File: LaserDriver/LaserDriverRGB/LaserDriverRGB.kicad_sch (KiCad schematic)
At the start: 15 parts

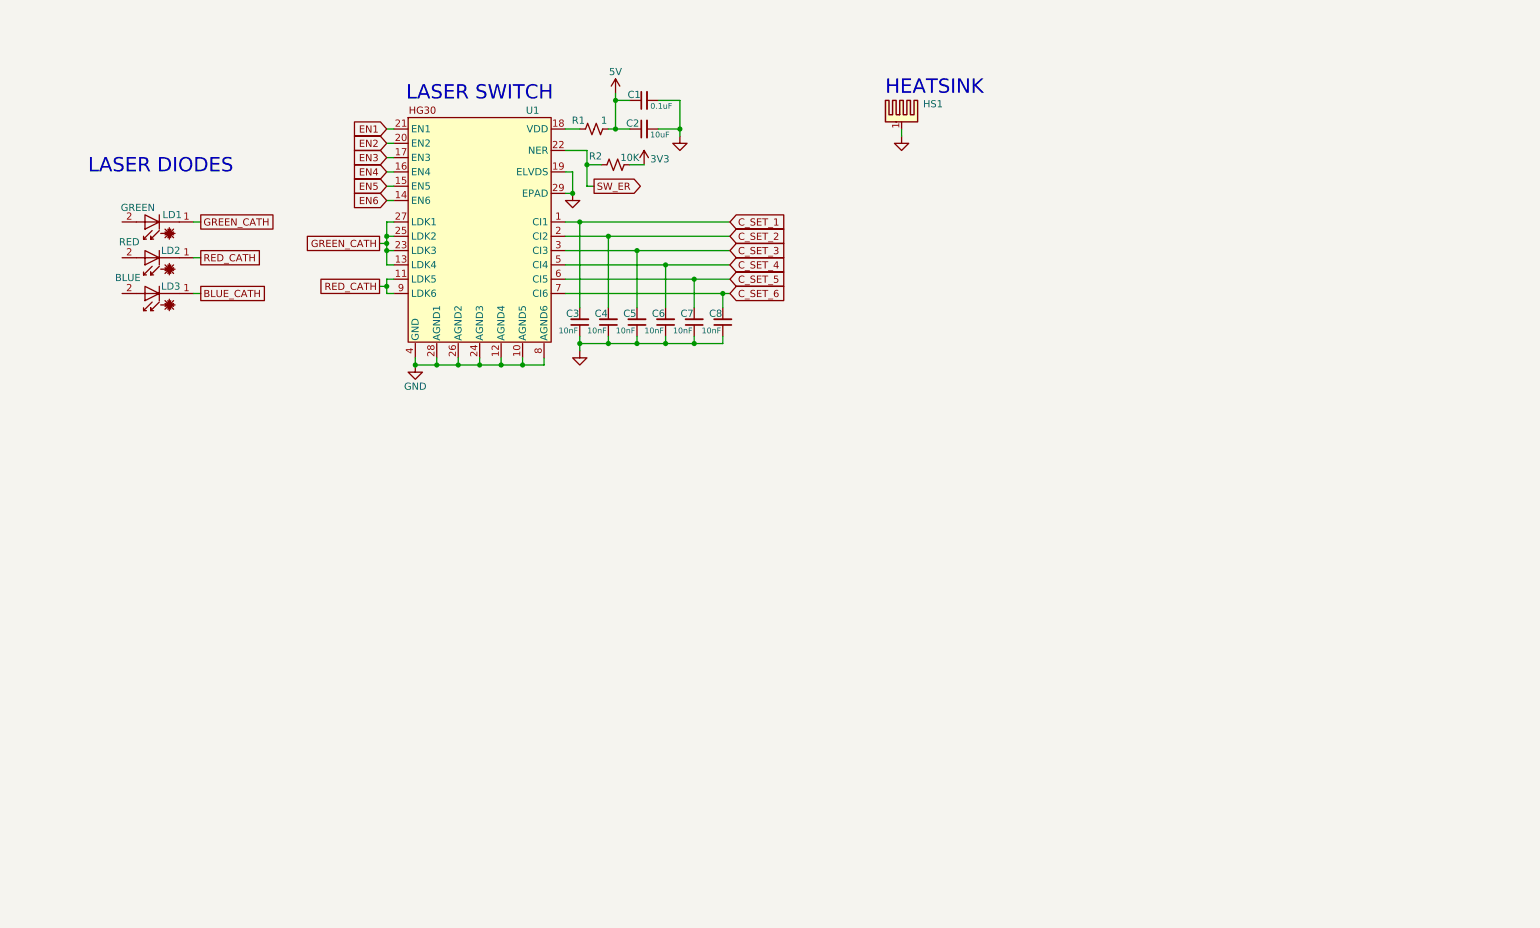
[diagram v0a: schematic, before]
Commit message: pcb chilling
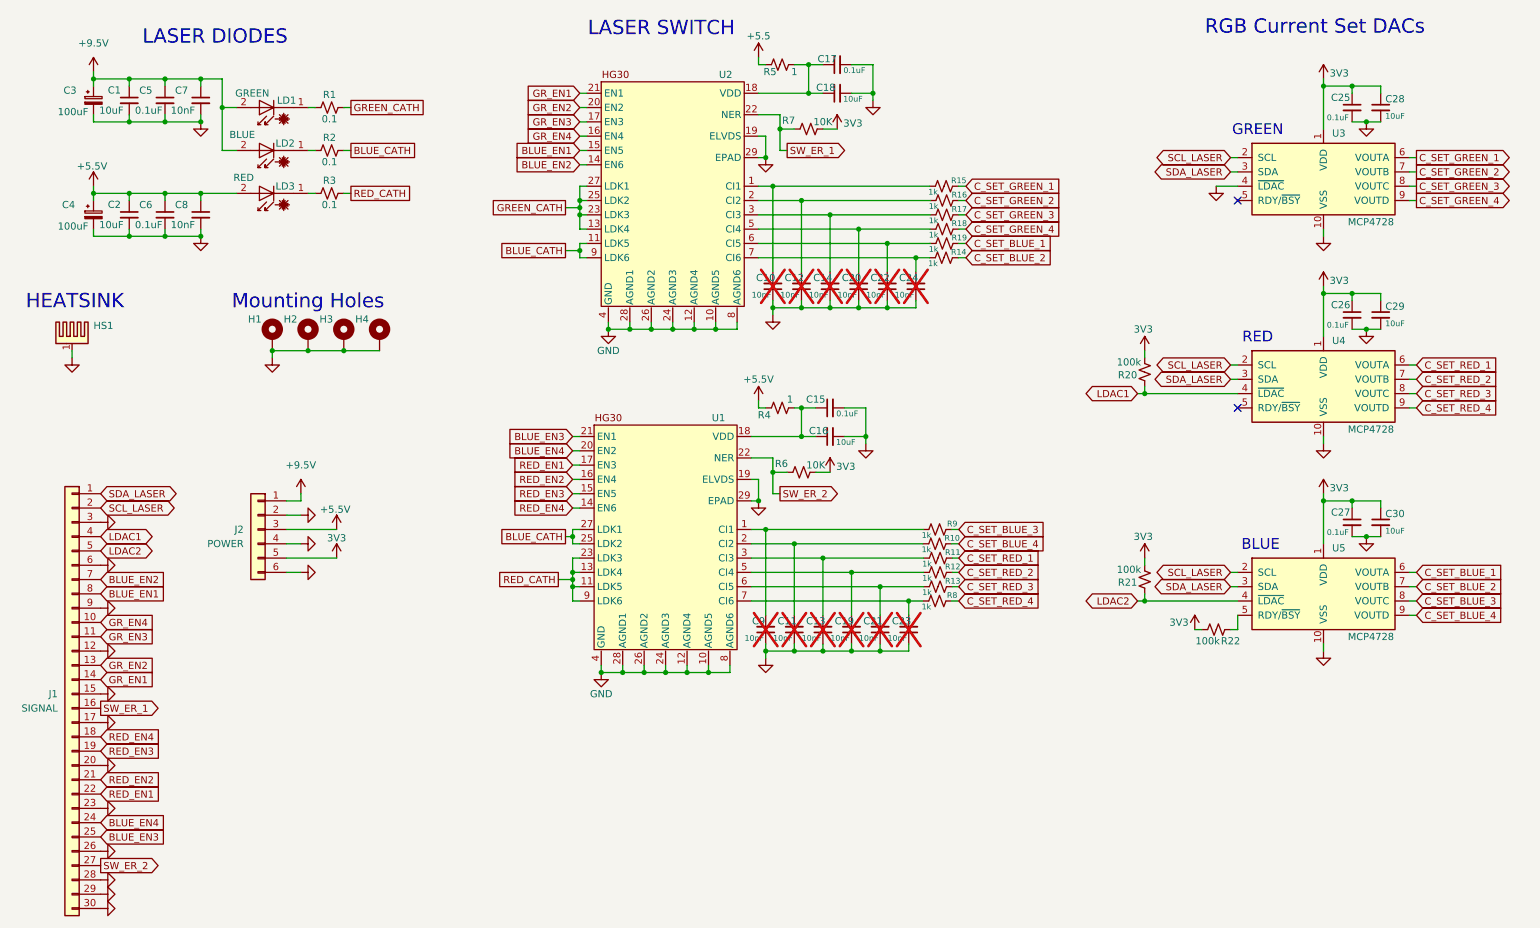
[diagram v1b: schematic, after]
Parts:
- added C1, C2: 100uF, Capacitor_THT:C_Radial_D5.0mm_H5.0mm_P2.00mm, symbol Device:C_Polarized_Small
- added C11, C13, C19, C21, C23, C9: 10nF, symbol Device:C_Small
- added C15, C25, C26, C27, C5, C6: 0.1uF, Capacitor_SMD:C_0603_1608Metric, symbol Device:C_Small
- added C16, C28, C29, C3, C30, C4: 10uF, Capacitor_SMD:C_0805_2012Metric, symbol Device:C_Small
- added C7, C8: 10nF, Capacitor_SMD:C_0603_1608Metric, symbol Device:C_Small
- added H1, H2, H3, H4: MountingHole_Pad, MountingHole:MountingHole_2.2mm_M2_DIN965_Pad, symbol Mechanical:MountingHole_Pad
- added J1: SIGNAL, PCM_SparkFun-Connector:FPC_1x30_P0.5mm_Horizontal_DualContact, symbol Connector_Generic:Conn_01x30
- added J2: POWER, Connector_Molex:Molex_DuraClik_502352-0600_1x06-1MP_P2.00mm_Horizontal, symbol Connector_Generic:Conn_01x06
- added R10, R11, R12, R13, R14, R15, R16, R17, R18, R19, R8, R9: 1k, Resistor_SMD:R_0603_1608Metric, symbol PCM_SparkFun-Resistor:R_Small
- added R2, R3: 0.1, Resistor_SMD:R_2512_6332Metric, symbol PCM_SparkFun-Resistor:R_Small
- added R20, R21, R22: 100k, Resistor_SMD:R_0603_1608Metric, symbol PCM_SparkFun-Resistor:R_Small
- added R4, R5: 1, Resistor_SMD:R_0603_1608Metric, symbol PCM_SparkFun-Resistor:R_Small
- added R6: 10K, Resistor_SMD:R_0603_1608Metric, symbol PCM_SparkFun-Resistor:R_Small
- added U1: (no value), Package_DFN_QFN:QFN-28-1EP_5x5mm_P0.5mm_EP2.7x2.7mm_ThermalVias, symbol ssi_IC:HG30
- added U3, U4, U5: MCP4728, Package_SO:MSOP-10_3x3mm_P0.5mm, symbol Analog_DAC:MCP4728
- C10: renamed from C3; now not fitted
- C12: renamed from C4; now not fitted
- C14: renamed from C5; now not fitted
- C17: renamed from C1; footprint (none) -> Capacitor_SMD:C_0603_1608Metric
- C18: renamed from C2; footprint (none) -> Capacitor_SMD:C_0805_2012Metric
- C20: renamed from C6; now not fitted
- C22: renamed from C7; now not fitted
- C24: renamed from C8; now not fitted
- HS1: footprint (none) -> TestPoint:TestPoint_Pad_4.0x4.0mm
- LD1: footprint (none) -> Connector_Molex:Molex_DuraClik_502352-0200_1x02-1MP_P2.00mm_Horizontal
- LD2: renamed from LD3; footprint (none) -> Connector_Molex:Molex_DuraClik_502352-0200_1x02-1MP_P2.00mm_Horizontal
- LD3: renamed from LD2; footprint (none) -> Connector_Molex:Molex_DuraClik_502352-0200_1x02-1MP_P2.00mm_Horizontal
- R1: value 1 -> 0.1; footprint PCM_SparkFun-Resistor:R_0603_1608Metric -> Resistor_SMD:R_2512_6332Metric
- R7: renamed from R2; footprint PCM_SparkFun-Resistor:R_0603_1608Metric -> Resistor_SMD:R_0603_1608Metric
- renumbered U1 to U2
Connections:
- net 3V3: now also C25.1, C26.1, C27.1, C28.1, C29.1, C30.1, J2.5 (Pin_5), R20.2, R21.2, R22.1, R6.2, U3.1 (VDD), U4.1 (VDD), U5.1 (VDD)
- net BLUE_CATH: now also U2.11 (LDK5), U2.9 (LDK6), R2.2, U1.25 (LDK2), U1.27 (LDK1); no longer LD2.1 (K)
- net GND: now also C1.2, C11.1, C13.1, C15.2, C16.2, C19.1, C2.2, C21.1, C23.1, C25.2, C26.2, C27.2, C28.2, C29.2, C3.2, C30.2, C4.2, C5.2, C6.2, C7.2, C8.2, C9.1, H1.1, H2.1, H3.1, H4.1, J1.12 (Pin_12), J1.15 (Pin_15), J1.17 (Pin_17), J1.20 (Pin_20), J1.23 (Pin_23), J1.26 (Pin_26), J1.28 (Pin_28), J1.29 (Pin_29), J1.3 (Pin_3), J1.30 (Pin_30), J1.6 (Pin_6), J1.9 (Pin_9), J2.2 (Pin_2), J2.4 (Pin_4), J2.6 (Pin_6), U1.10 (AGND5), U1.12 (AGND4), U1.19 (ELVDS), U1.24 (AGND3), U1.26 (AGND2), U1.28 (AGND1), U1.29 (EPAD), U1.4 (GND), U1.8 (AGND6), U3.10 (VSS), U3.4 (~{LDAC}), U4.10 (VSS), U5.10 (VSS)
- net GREEN_CATH: now also R1.2; no longer LD1.1 (K)
- net RED_CATH: now also R3.2, U1.11 (LDK5), U1.13 (LDK4), U1.23 (LDK3), U1.9 (LDK6); no longer LD3.1 (K), U2.11 (LDK5), U2.9 (LDK6)
- net at U2.18 (VDD): now also C17.1, C18.1, R5.1; no longer R1.1
- net +9.5V: now reaches LD2.2 (A)
- net +9.5V: now also LD1.2 (A), C1.1, C3.1, C5.1, C7.1, J2.1 (Pin_1)
- net +5.5V: now reaches LD3.2 (A)
- net +5.5V: now also C2.1, C4.1, C6.1, C8.1, J2.3 (Pin_3), R4.1
- removed net 5V: C17.1, C18.1, R1.2
- net C_SET_1: no longer names the net of C10.2, U2.1 (CI1)
- net C_SET_1: now also R15.1
- net C_SET_2: no longer names the net of C12.2, U2.2 (CI2)
- net C_SET_2: now also R16.1
- net C_SET_3: no longer names the net of C14.2, U2.3 (CI3)
- net C_SET_3: now also R17.1
- net C_SET_4: no longer names the net of C20.2, U2.5 (CI4)
- net C_SET_4: now also R18.1
- net C_SET_5: no longer names the net of C22.2, U2.6 (CI5)
- net C_SET_5: now also R19.1
- net C_SET_6: no longer names the net of C24.2, U2.7 (CI6)
- net C_SET_6: now also R14.1
- net EN1 renamed GR_EN1
- net GR_EN1: now also J1.14 (Pin_14)
- net EN2 renamed GR_EN2
- net GR_EN2: now also J1.13 (Pin_13)
- net EN3 renamed GR_EN3
- net GR_EN3: now also J1.11 (Pin_11)
- net EN4 renamed GR_EN4
- net GR_EN4: now also J1.10 (Pin_10)
- net EN5 renamed BLUE_EN1
- net BLUE_EN1: now also J1.8 (Pin_8)
- net EN6 renamed BLUE_EN2
- net BLUE_EN2: now also J1.7 (Pin_7)
- net SW_ER renamed SW_ER_1
- net SW_ER_1: now also J1.16 (Pin_16)
- new net: C11.2, R10.1, U1.2 (CI2)
- new net: C13.2, R11.1, U1.3 (CI3)
- new net: C9.2, R9.1, U1.1 (CI1)
- new net: C15.1, C16.1, R4.2, U1.18 (VDD)
- new net: LD2.1 (K), R2.1
- new net: LD1.1 (K), R1.1
- new net: C19.2, R12.1, U1.5 (CI4)
- new net: C23.2, R8.1, U1.7 (CI6)
- new net: C21.2, R13.1, U1.6 (CI5)
- new net: R22.2, U5.5 (RDY/~{BSY})
- new net: LD3.1 (K), R3.1
- new net +5.5: R5.2
- new net BLUE_EN3: J1.25 (Pin_25), U1.21 (EN1)
- new net BLUE_EN4: J1.24 (Pin_24), U1.20 (EN2)
- new net C_SET_BLUE_1: R19.2, U5.6 (VOUTA)
- new net C_SET_BLUE_2: R14.2, U5.7 (VOUTB)
- new net C_SET_BLUE_3: R9.2, U5.8 (VOUTC)
- new net C_SET_BLUE_4: R10.2, U5.9 (VOUTD)
- new net C_SET_GREEN_1: R15.2, U3.6 (VOUTA)
- new net C_SET_GREEN_2: R16.2, U3.7 (VOUTB)
- new net C_SET_GREEN_3: R17.2, U3.8 (VOUTC)
- new net C_SET_GREEN_4: R18.2, U3.9 (VOUTD)
- new net C_SET_RED_1: R11.2, U4.6 (VOUTA)
- new net C_SET_RED_2: R12.2, U4.7 (VOUTB)
- new net C_SET_RED_3: R13.2, U4.8 (VOUTC)
- new net C_SET_RED_4: R8.2, U4.9 (VOUTD)
- new net LDAC1: J1.4 (Pin_4), R20.1, U4.4 (~{LDAC})
- new net LDAC2: J1.5 (Pin_5), R21.1, U5.4 (~{LDAC})
- new net RED_EN1: J1.22 (Pin_22), U1.17 (EN3)
- new net RED_EN2: J1.21 (Pin_21), U1.16 (EN4)
- new net RED_EN3: J1.19 (Pin_19), U1.15 (EN5)
- new net RED_EN4: J1.18 (Pin_18), U1.14 (EN6)
- new net SCL_LASER: J1.2 (Pin_2), U3.2 (SCL), U4.2 (SCL), U5.2 (SCL)
- new net SDA_LASER: J1.1 (Pin_1), U3.3 (SDA), U4.3 (SDA), U5.3 (SDA)
- new net SW_ER_2: J1.27 (Pin_27), R6.1, U1.22 (NER)
- no-connect marks 0 -> 2
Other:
- note added: "BLUE"
- note added: "GREEN"
- note added: "Mounting Holes"
- note added: "RED"
- note added: "RGB Current Set DACs"
- moved on the sheet: C17, C18, HS1, LD1, LD2, LD3, R7, U2
